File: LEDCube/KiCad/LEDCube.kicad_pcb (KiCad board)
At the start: 2 copper layers, 70 x 50 mm, 9 parts, among them J1 BARREL_JACK, J2 ICSP HEADER, J3 TO_ANODES, J4 TO_CATHODES, U1 ATMEGA16-16PU, U2 LM7805, U3 ULN2803A

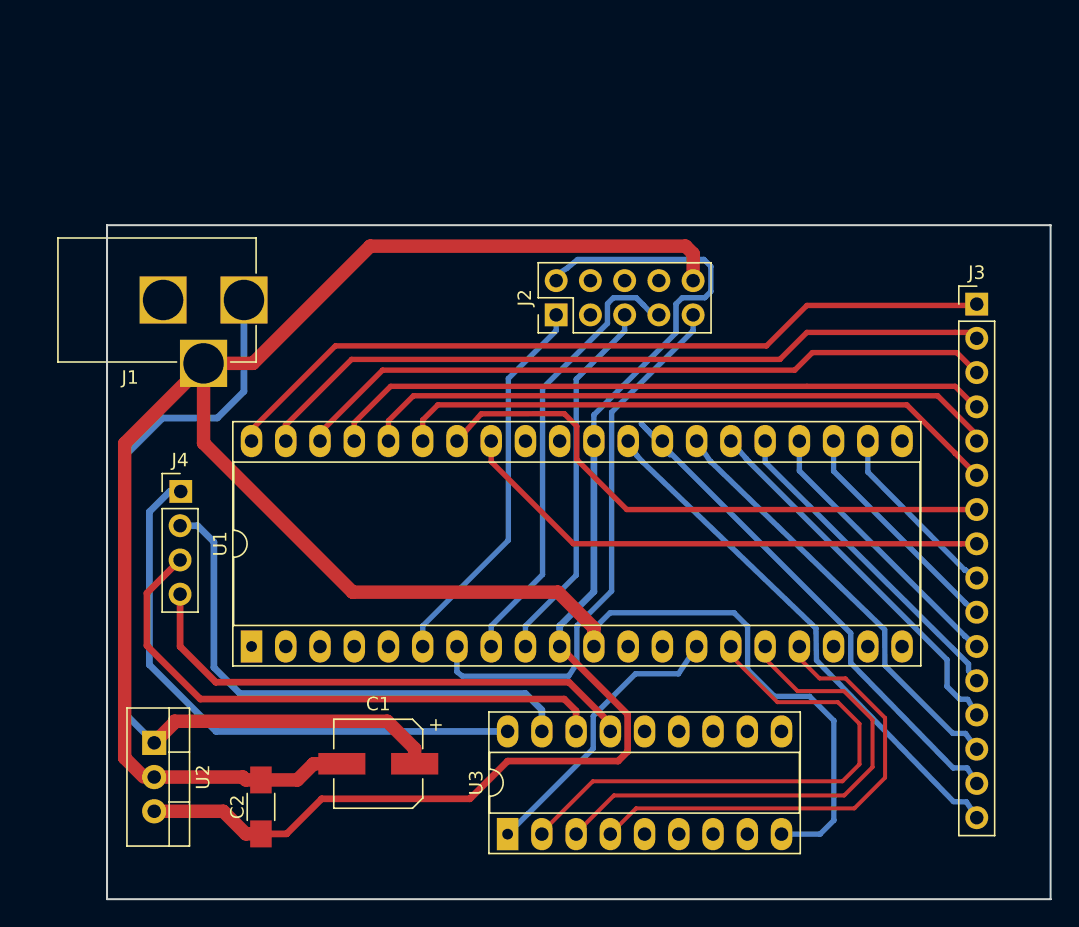
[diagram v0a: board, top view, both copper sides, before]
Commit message: Minor changes
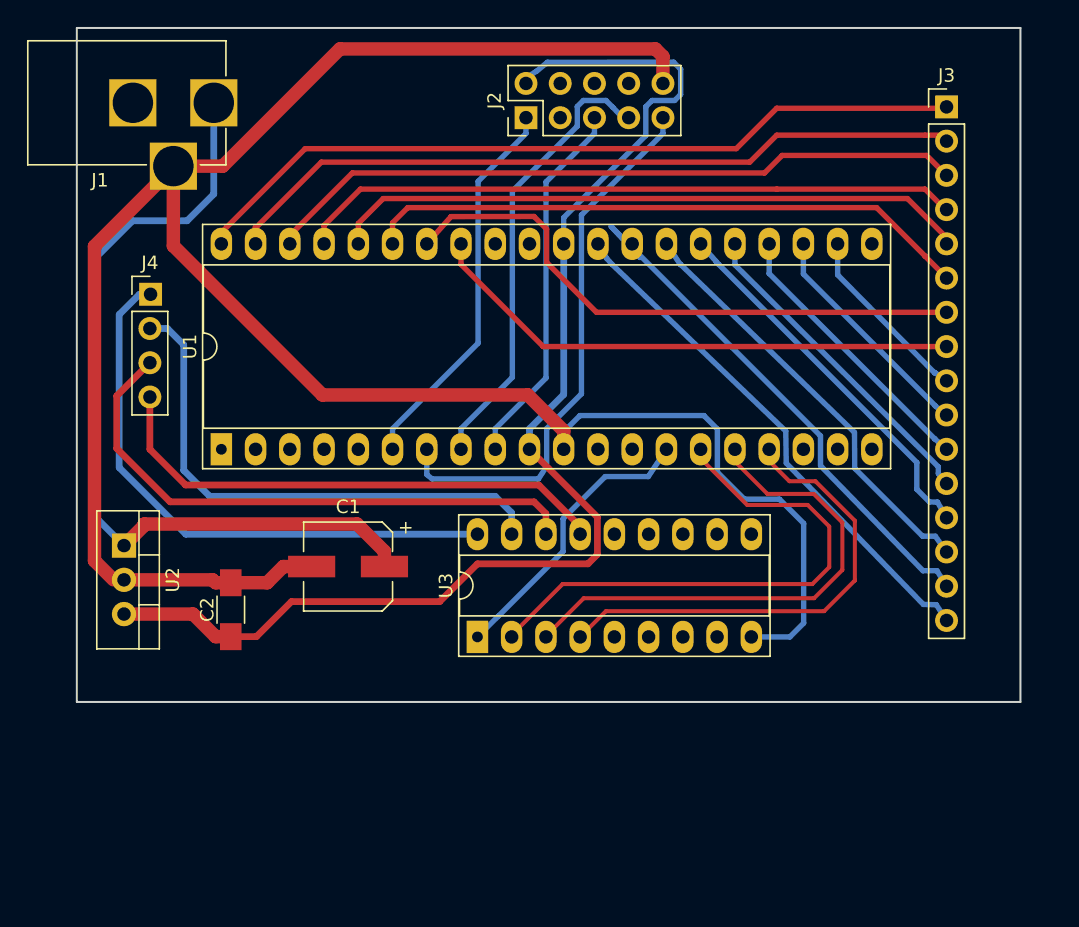
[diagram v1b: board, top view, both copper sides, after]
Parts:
- moved U2 14.8 mm to (70.7, 80.4)
- moved U3 14.8 mm to (96.9, 87.1)
- moved J1 14.8 mm to (77.3, 47.5)
- moved J2 14.8 mm to (100.5, 48.6)
- moved J3 14.8 mm to (131.7, 47.8)
- moved C1 14.8 mm to (87.3, 81.9)
- moved C2 14.8 mm to (78.6, 85.1)
- moved J4 14.8 mm to (72.6, 61.7)
- moved U1 14.8 mm to (77.9, 73.2)
